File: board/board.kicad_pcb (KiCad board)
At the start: 2 copper layers, 21 x 13 mm, 1 part

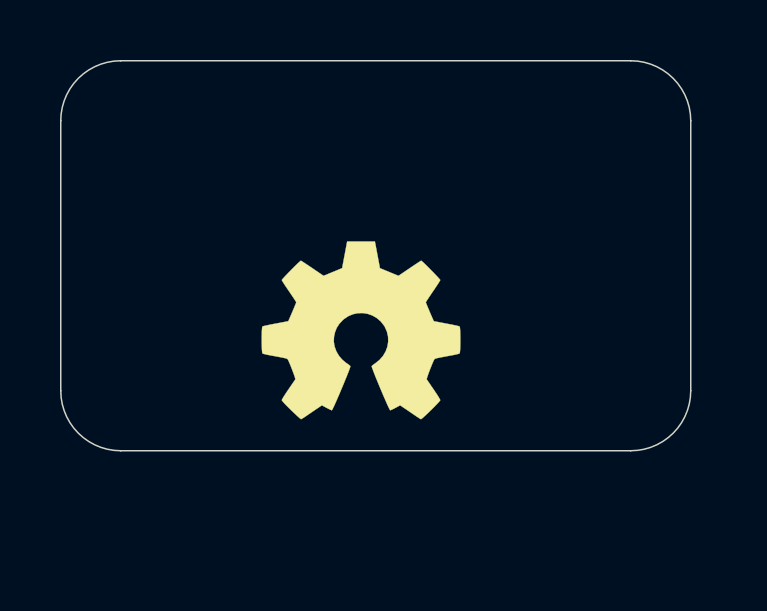
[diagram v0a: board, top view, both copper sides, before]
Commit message: initial
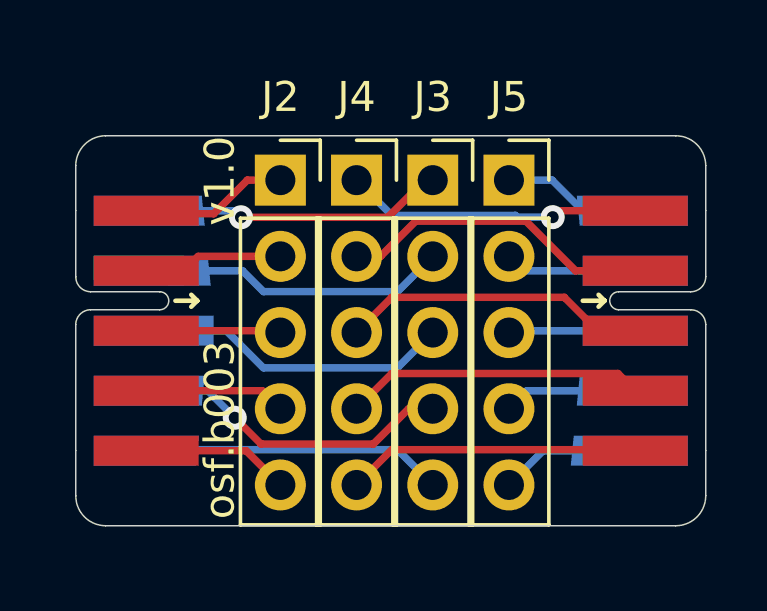
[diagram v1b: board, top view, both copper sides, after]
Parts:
- removed LOGO1: Logo_Open_Hardware_Small, Symbol:OSHW-Symbol_6.7x6mm_SilkScreen
- added J1: Conn_01x10_Male, on_edge:on_edge_2x05_device, F.Cu at (140.5, 99.0)
- added J2: Conn_01x05_Male, Connector_PinSocket_2.54mm:PinSocket_1x05_P2.54mm_Vertical, F.Cu at (147.3, 94.0)
- added J3: Conn_01x05_Male, Connector_PinSocket_2.54mm:PinSocket_1x05_P2.54mm_Vertical, F.Cu at (152.4, 94.0)
- added J4: Conn_01x05_Male, Connector_PinSocket_2.54mm:PinSocket_1x05_P2.54mm_Vertical, F.Cu at (149.9, 94.0)
- added J5: Conn_01x05_Male, Connector_PinSocket_2.54mm:PinSocket_1x05_P2.54mm_Vertical, F.Cu at (154.9, 94.0)
- added J6: Conn_01x10_Male, on_edge:on_edge_2x05_host, F.Cu at (161.5, 99.0)
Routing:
- net Net-(J1-Pad8): track 0.00 -> 10.8 mm
- net Net-(J1-Pad9): track 0.00 -> 10.7 mm, vias 0 -> 1
- net Net-(J1-Pad7): track 0.00 -> 10.6 mm
- net Net-(J1-Pad6): track 0.00 -> 10.1 mm, vias 0 -> 1
- net Net-(J1-Pad10): track 0.00 -> 10.1 mm
- net Net-(J4-Pad4): track 0.00 -> 10.0 mm
- net Net-(J4-Pad1): track 0.00 -> 9.89 mm, vias 0 -> 1
- net Net-(J4-Pad5): track 0.00 -> 9.79 mm
- net Net-(J4-Pad2): track 0.00 -> 9.21 mm
- net Net-(J4-Pad3): track 0.00 -> 8.99 mm
- net Net-(J1-Pad1): track 0.00 -> 4.98 mm
- net Net-(J1-Pad5): track 0.00 -> 4.94 mm
- net Net-(J1-Pad4): track 0.00 -> 4.72 mm
- net Net-(J5-Pad2): track 0.00 -> 4.66 mm
- net Net-(J5-Pad1): track 0.00 -> 4.58 mm
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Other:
- outline, holes or cut-outs redrawn
- copper layers 2 -> 4
- rule pad_to_mask_clearance: 0 -> 0.051
- board text added: "osf.b003"
- board text added: "v1.0"
